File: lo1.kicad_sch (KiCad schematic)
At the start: 1 part

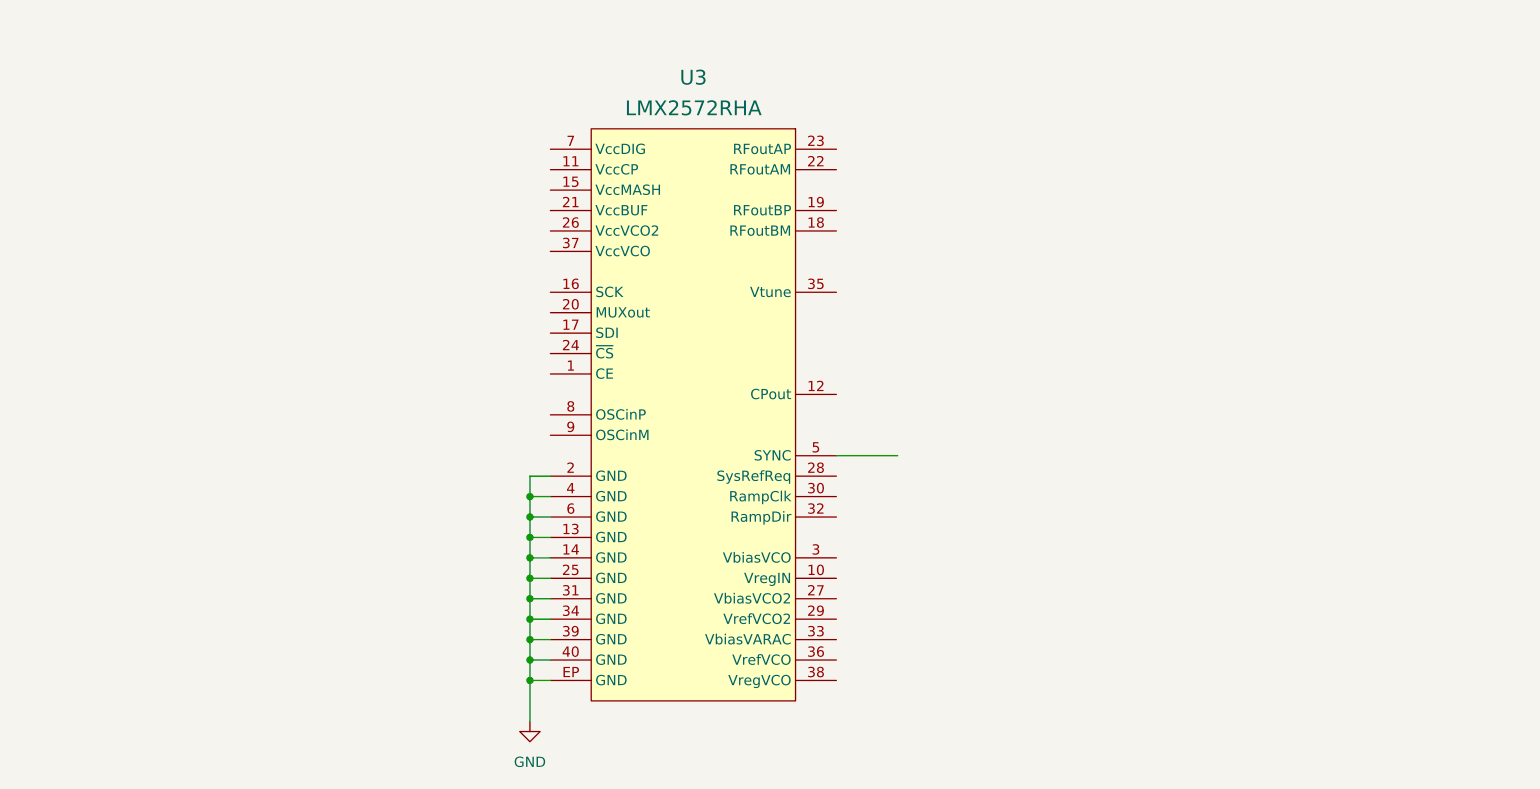
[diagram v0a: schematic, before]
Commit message: lo1 schematic
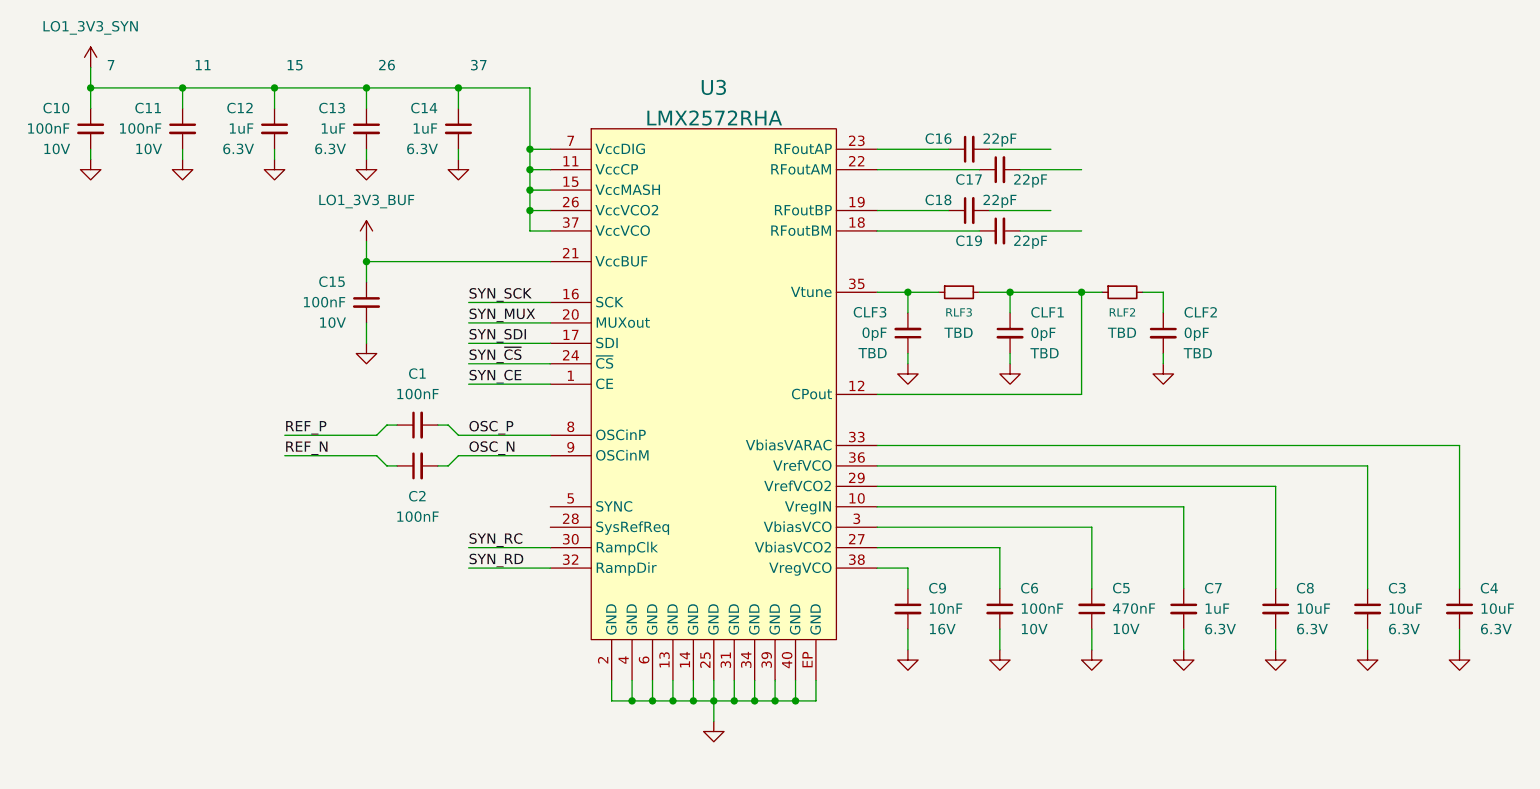
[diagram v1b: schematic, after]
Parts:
- added C1, C10, C11, C15, C2, C6: 100nF, ar_passives:C_0402, symbol #bt-db:capacitor/CAPC-00573
- added C12, C13, C14, C7: 1uF, ar_passives:C_0402, symbol #bt-db:capacitor/CAPC-00622
- added C16, C17, C18, C19: 22pF, ar_passives:C_0201, symbol #bt-db:capacitor/CAPC-00021
- added C3, C4, C8: 10uF, ar_passives:C_0402, symbol #bt-db:capacitor/CAPC-00667
- added C5: 470nF, ar_passives:C_0402, symbol #bt-db:capacitor/CAPC-00613
- added C9: 10nF, ar_passives:C_0402, symbol #bt-db:capacitor/CAPC-00514
- added CLF1: 0pF, ar_passives:C_0603, symbol #bt-db:capacitor/CAPC-00674
- added CLF2, CLF3: 0pF, ar_passives:C_0402, symbol #bt-db:capacitor/CAPC-00415
- added RLF2, RLF3: TBD, ar_passives:R_0402, symbol #bt-db:resistor/RESI-00693
- U3: footprint ar_discrete:QFN40 -> ar_ic:QFN40
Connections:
- net GND: now also C10.2, C11.2, C12.2, C13.2, C14.2, C15.2, C3.2, C4.2, C5.1, C6.2, C7.2, C8.2, C9.2, CLF1.2, CLF2.2, CLF3.1
- net SYN_CE: now reaches U3.1 (CE)
- net at U3.10 (VregIN): now also C7.1
- net LO1_3V3_SYN: now reaches U3.11 (VccCP)
- net LO1_3V3_SYN: now also U3.15 (VccMASH), U3.26 (VccVCO2), U3.37 (VccVCO), U3.7 (VccDIG), C10.1, C11.1, C12.1, C13.1, C14.1
- net at U3.12 (CPout): now also CLF1.1, RLF2.1, RLF3.2
- net SYN_SCK: now reaches U3.16 (SCK)
- net SYN_SDI: now reaches U3.17 (SDI)
- net at U3.18 (RFoutBM): now also C19.1
- net at U3.19 (RFoutBP): now also C18.1
- net SYN_MUX: now reaches U3.20 (MUXout)
- net LO1_3V3_BUF: now reaches U3.21 (VccBUF)
- net LO1_3V3_BUF: now also C15.1
- net at U3.22 (RFoutAM): now also C17.1
- net at U3.23 (RFoutAP): now also C16.1
- net SYN_~{CS}: now reaches U3.24 (~{CS})
- net at U3.27 (VbiasVCO2): now also C6.1
- net at U3.29 (VrefVCO2): now also C8.1
- net at U3.3 (VbiasVCO): now also C5.2
- net SYN_RC: now reaches U3.30 (RampClk)
- net SYN_RD: now reaches U3.32 (RampDir)
- net at U3.33 (VbiasVARAC): now also C4.1
- net at U3.35 (Vtune): now also CLF3.2, RLF3.1
- net at U3.36 (VrefVCO): now also C3.1
- net at U3.38 (VregVCO): now also C9.1
- net OSC_P: now reaches U3.8 (OSCinP)
- net OSC_P: now also C1.2
- net OSC_N: now reaches U3.9 (OSCinM)
- net OSC_N: now also C2.2
- new net: CLF2.1, RLF2.2
- new net REF_N: C2.1
- new net REF_P: C1.1
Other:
- note added: "11"
- note added: "15"
- note added: "26"
- note added: "37"
- note added: "7"
